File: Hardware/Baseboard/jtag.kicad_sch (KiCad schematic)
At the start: 5 parts, among them J3 USB_C_Receptacle_USB2.0_16P, U1 93LCxxC, U3 FT2232HL

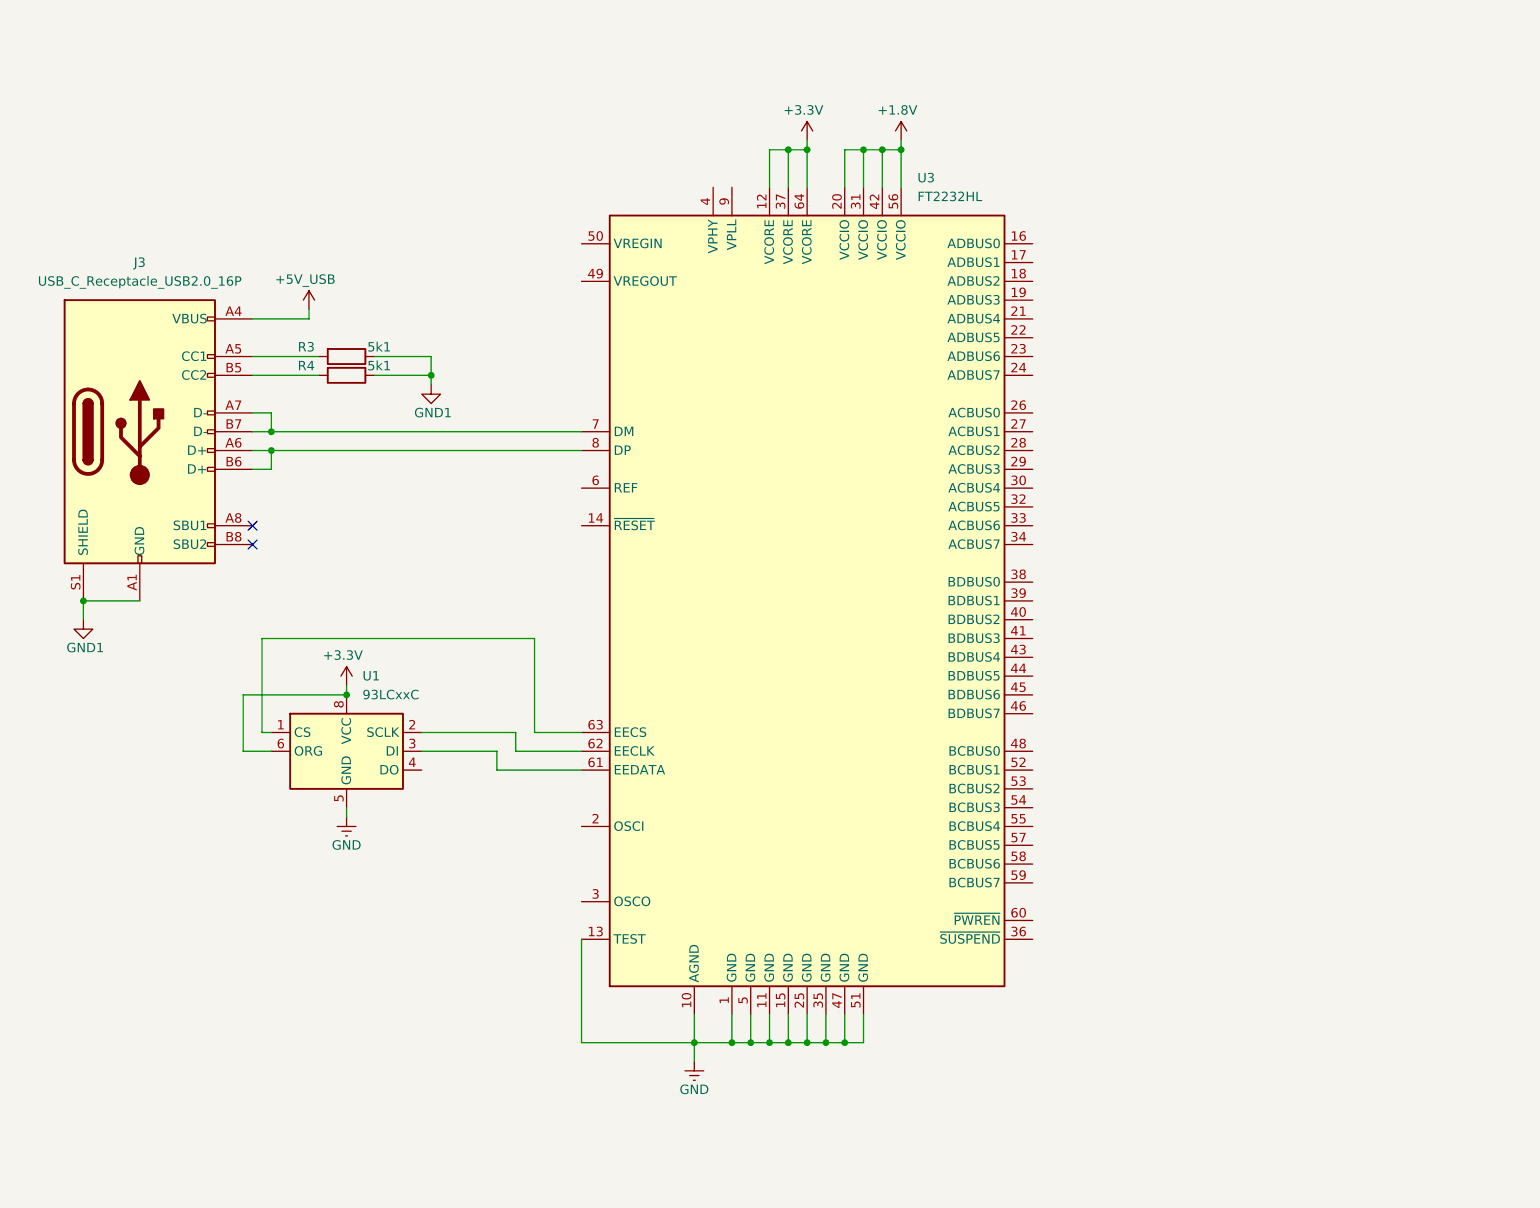
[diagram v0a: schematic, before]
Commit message: Baseboard: JTAG
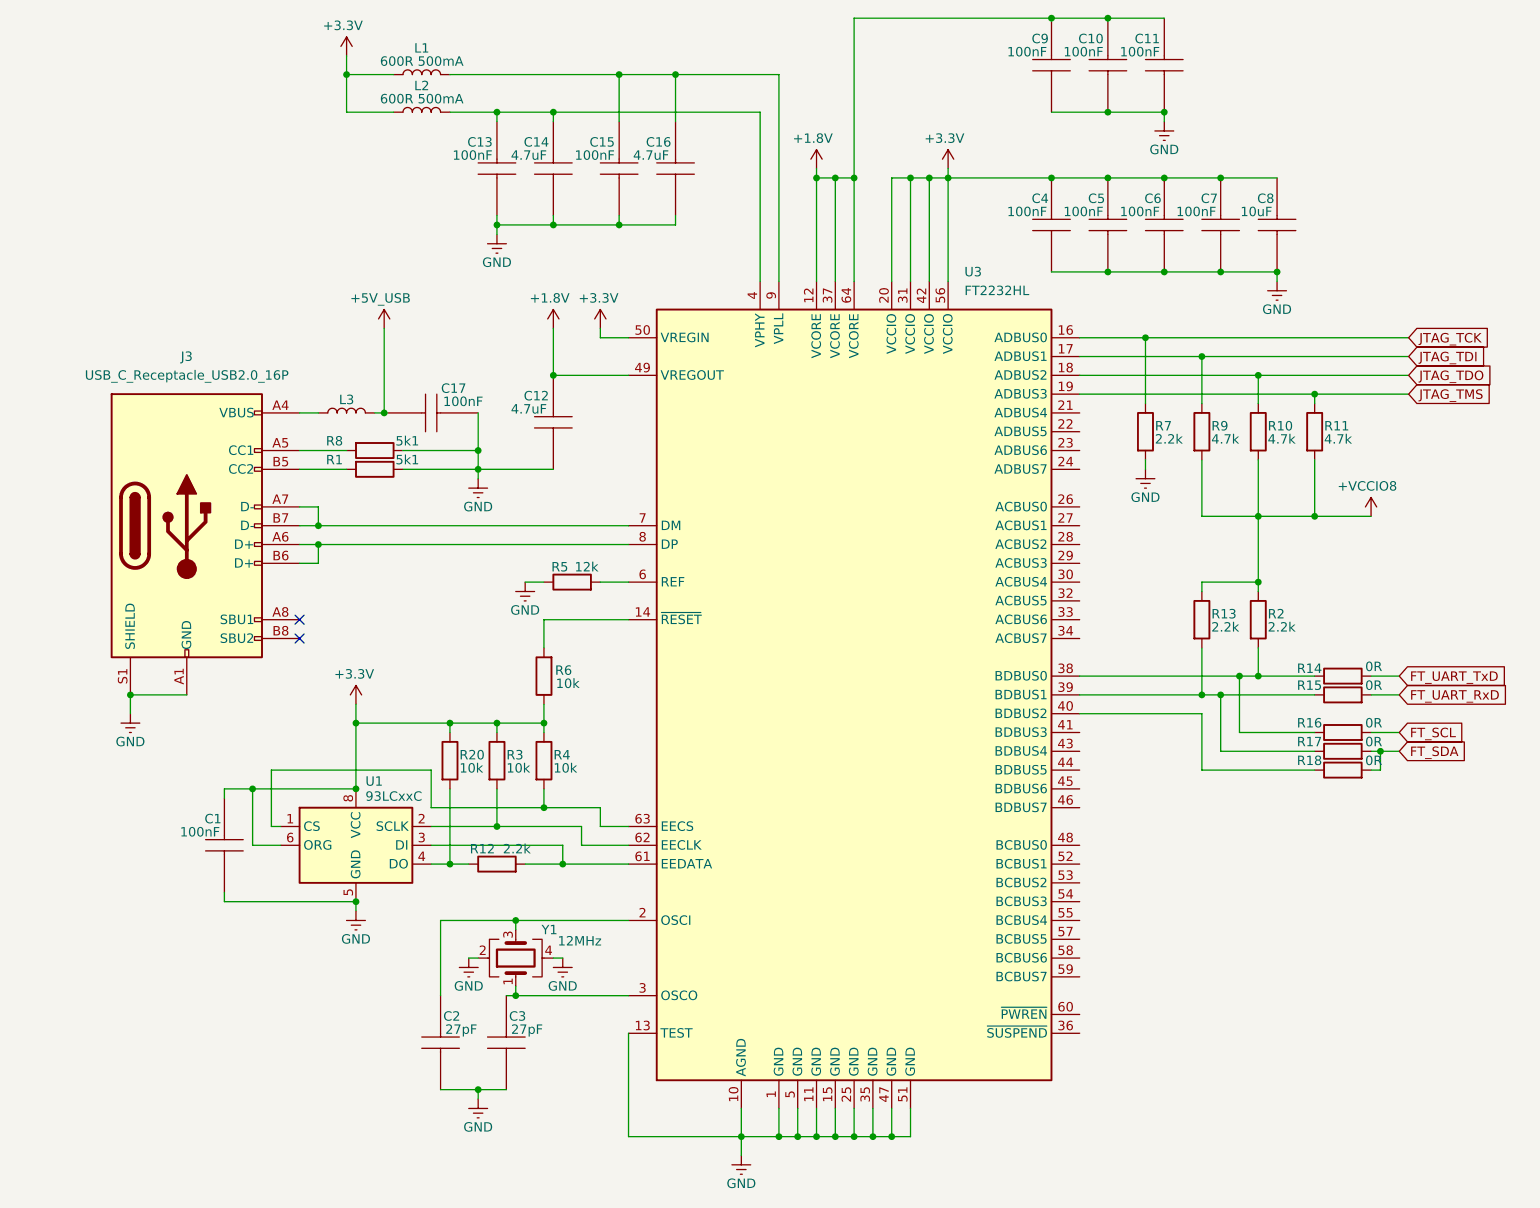
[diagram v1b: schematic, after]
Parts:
- added C1, C10, C11, C13, C15, C17, C4, C5, C6, C7, C9: 100nF, Capacitor_SMD:C_0402_1005Metric, symbol RA8M1:885012205092
- added C12, C14, C16: 4.7uF, Capacitor_SMD:C_0402_1005Metric, symbol RA8M1:885012205092
- added C2, C3: 27pF, Capacitor_SMD:C_0402_1005Metric, symbol RA8M1:885012205092
- added C8: 10uF, Capacitor_SMD:C_0402_1005Metric, symbol RA8M1:885012205092
- added L1, L2, L3: 600R 500mA, symbol Device:L
- added R1, R8: 5k1, Resistor_SMD:R_0402_1005Metric, symbol Device:R
- added R10, R11, R9: 4.7k, Resistor_SMD:R_0402_1005Metric, symbol Device:R
- added R12, R13, R2, R7: 2.2k, Resistor_SMD:R_0402_1005Metric, symbol Device:R
- added R14, R15, R16, R17, R18: 0R, Resistor_SMD:R_0402_1005Metric, symbol Device:R
- added R20, R6: 10k, Resistor_SMD:R_0402_1005Metric, symbol Device:R
- added R5: 12k, Resistor_SMD:R_0402_1005Metric, symbol Device:R
- added Y1: 12MHz, Crystal:Crystal_SMD_3225-4Pin_3.2x2.5mm, symbol Device:Crystal_GND24
- R3, R4: value 5k1 -> 10k; footprint Resistor_SMD:R_0805_2012Metric -> Resistor_SMD:R_0402_1005Metric; MPN 560112120019 -> 560112110020
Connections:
- net +1.8V: now also U3.12 (VCORE), U3.37 (VCORE), U3.49 (VREGOUT), U3.64 (VCORE), C10.2, C11.2, C12.2, C9.2; no longer U3.20 (VCCIO), U3.31 (VCCIO), U3.42 (VCCIO), U3.56 (VCCIO)
- net +3.3V: now also R3.1, R4.1, U3.20 (VCCIO), U3.31 (VCCIO), U3.42 (VCCIO), U3.50 (VREGIN), U3.56 (VCCIO), C1.2, C4.2, C5.2, C6.2, C7.2, C8.2, L1.1, L2.1, R20.1, R6.1; no longer U3.12 (VCORE), U3.37 (VCORE), U3.64 (VCORE)
- net +5V_USB: now also C17.1, L3.2; no longer J3.A4 (VBUS), J3.A9 (VBUS), J3.B4 (VBUS), J3.B9 (VBUS)
- net GND: now also J3.A1 (GND), J3.A12 (GND), J3.B1 (GND), J3.B12 (GND), J3.S1 (SHIELD), C1.1, C10.1, C11.1, C12.1, C13.1, C14.1, C15.1, C16.1, C17.2, C2.1, C3.1, C4.1, C5.1, C6.1, C7.1, C8.1, C9.1, R1.1, R5.1, R7.2, R8.1, Y1.2, Y1.4
- net at R4.2: now also U1.1 (CS), U3.63 (EECS); no longer J3.B5 (CC2)
- net at U1.2 (SCLK), U3.62 (EECLK): now also R3.2
- net at U1.3 (DI), U3.61 (EEDATA): now also R12.2
- net at U1.4 (DO): now also R12.1, R20.2
- net at U3.14 (~{RESET}): now also R6.2
- net JTAG_TCK: now reaches U3.16 (ADBUS0)
- net JTAG_TCK: now also R7.1
- net JTAG_TDI: now reaches U3.17 (ADBUS1)
- net JTAG_TDI: now also R9.1
- net JTAG_TDO: now reaches U3.18 (ADBUS2)
- net JTAG_TDO: now also R10.1
- net JTAG_TMS: now reaches U3.19 (ADBUS3)
- net JTAG_TMS: now also R11.1
- net at U3.2 (OSCI): now also C2.2, Y1.3
- net at U3.3 (OSCO): now also C3.2, Y1.1
- net at U3.38 (BDBUS0): now also R14.1, R16.1, R2.2
- net at U3.39 (BDBUS1): now also R13.2, R15.1, R17.1
- net at U3.4 (VPHY): now also C13.2, C14.2, L2.2
- net at U3.40 (BDBUS2): now also R18.1
- net at U3.6 (REF): now also R5.2
- net at U3.9 (VPLL): now also C15.2, C16.2, L1.2
- net at J3.A5 (CC1): now also R8.2; no longer R3.2
- removed net GND1: J3.A1 (GND), J3.A12 (GND), J3.B1 (GND), J3.B12 (GND), J3.S1 (SHIELD), R3.1, R4.1
- new net: J3.B5 (CC2), R1.2
- new net: J3.A4 (VBUS), J3.A9 (VBUS), J3.B4 (VBUS), J3.B9 (VBUS), L3.1
- new net +VCCIO8: R10.2, R11.2, R13.1, R2.1, R9.2
- new net FT_SCL: R16.2
- new net FT_SDA: R17.2, R18.2
- new net FT_UART_RxD: R15.2
- new net FT_UART_TxD: R14.2
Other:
- moved on the sheet: J3, U1, U3
